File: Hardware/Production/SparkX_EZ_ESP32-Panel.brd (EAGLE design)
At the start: 187.2 x 95.5 mm, 1506 parts, among them Q1 MBT3904DW1T1, Q10 MBT3904DW1T1, Q11 MBT3904DW1T1, Q12 MBT3904DW1T1, Q13 MBT3904DW1T1, Q14 MBT3904DW1T1, Q15 MBT3904DW1T1, Q16 MBT3904DW1T1, Q17 MBT3904DW1T1, Q18 MBT3904DW1T1, Q19 MBT3904DW1T1, Q2 MBT3904DW1T1, Q20 MBT3904DW1T1, Q3 MBT3904DW1T1, Q4 MBT3904DW1T1, Q5 MBT3904DW1T1, Q6 MBT3904DW1T1, Q7 MBT3904DW1T1, Q8 MBT3904DW1T1, Q9 MBT3904DW1T1, U1 MIC5219 3.3V, U10 W25QXX128MBIT-6X5-SKINNY_CENT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, U11 CP2102N, U12 MIC5219 3.3V, U13 ESP32, U14 W25QXX128MBIT-6X5-SKINNY_CENT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, U15 CP2102N, U16 MIC5219 3.3V, U17 ESP32, U18 W25QXX128MBIT-6X5-SKINNY_CENT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, U19 CP2102N, U2 ESP32, U20 MIC5219 3.3V, U21 ESP32, U22 W25QXX128MBIT-6X5-SKINNY_CENT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, U23 CP2102N, U24 MIC5219 3.3V, U25 ESP32, U26 W25QXX128MBIT-6X5-SKINNY_CENT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, U27 CP2102N, U28 MIC5219 3.3V, U29 ESP32, U3 W25QXX128MBIT-6X5-SKINNY_CENT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, U30 W25QXX128MBIT-6X5-SKINNY_CENT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, U31 CP2102N, U32 MIC5219 3.3V, U33 ESP32, U34 W25QXX128MBIT-6X5-SKINNY_CENT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, U35 CP2102N, U36 MIC5219 3.3V, U37 ESP32, U38 W25QXX128MBIT-6X5-SKINNY_CENT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, U39 CP2102N, U4 CP2102N, U40 MIC5219 3.3V, U41 ESP32, U42 W25QXX128MBIT-6X5-SKINNY_CENT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, U43 CP2102N, U44 MIC5219 3.3V, U45 ESP32, U46 W25QXX128MBIT-6X5-SKINNY_CENT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, U47 CP2102N, U48 MIC5219 3.3V, U49 ESP32, U5 ESP32, U50 W25QXX128MBIT-6X5-SKINNY_CENT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, U51 CP2102N, U52 MIC5219 3.3V, U53 ESP32, U54 W25QXX128MBIT-6X5-SKINNY_CENT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, U55 CP2102N, U56 MIC5219 3.3V, U57 ESP32, U58 W25QXX128MBIT-6X5-SKINNY_CENT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, U59 CP2102N, U6 W25QXX128MBIT-6X5-SKINNY_CENT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, U60 MIC5219 3.3V, U61 ESP32, U62 W25QXX128MBIT-6X5-SKINNY_CENT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, U63 CP2102N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

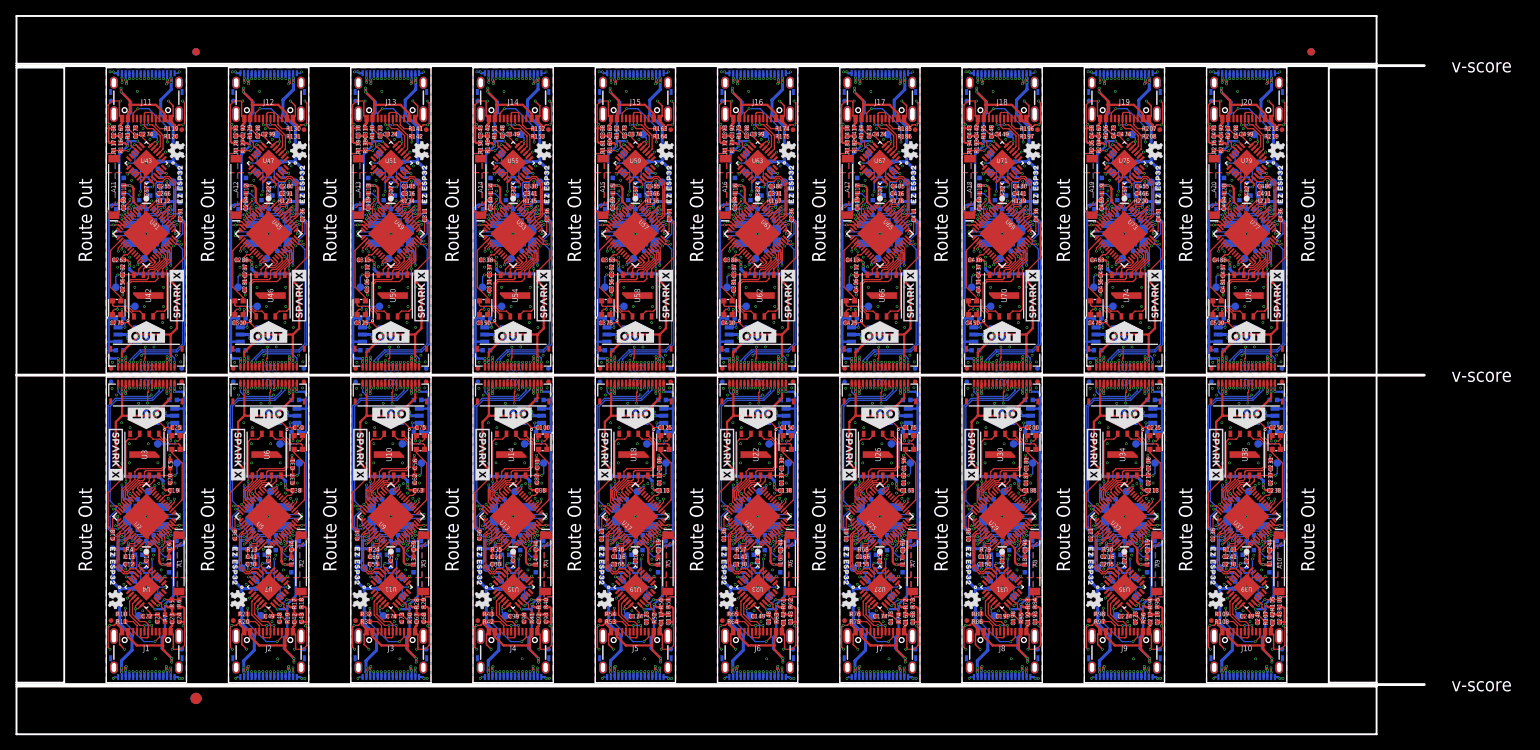
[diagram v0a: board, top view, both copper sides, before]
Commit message: Post-review updates
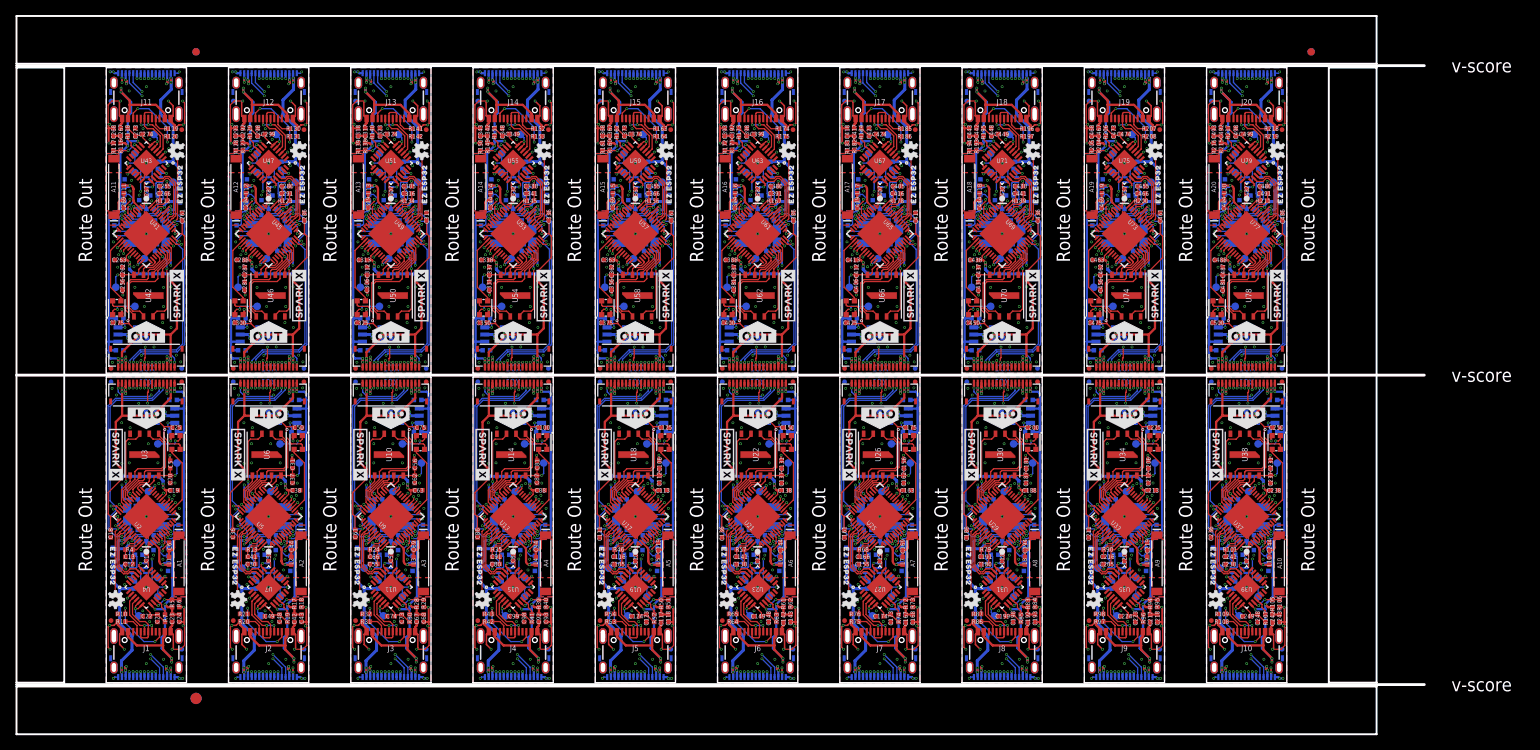
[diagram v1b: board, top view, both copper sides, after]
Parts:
- C1, C122, C147, C172, C197, C222, C247, C272, C297, C322, C347, C372, C397, C422, C447, C47, C472, C497, C72, C97: value 0.1uF -> 2.2uF
- moved C204 1.17 mm to (139.6, 20.5)
- moved C229 1.17 mm to (155.9, 20.5)
- moved C179 1.17 mm to (123.4, 20.5)
- moved C329 1.17 mm to (49.8, 61.3)
- moved C354 1.17 mm to (66.1, 61.3)
- moved C379 1.17 mm to (82.4, 61.3)
- moved C404 1.17 mm to (98.6, 61.3)
- moved C429 1.17 mm to (114.9, 61.3)
- moved C279 1.17 mm to (17.3, 61.3)
- moved C29 1.17 mm to (25.8, 20.5)
- moved C254 1.17 mm to (1.08, 61.3)
- moved C11 1.17 mm to (9.59, 20.5)
- moved C304 1.17 mm to (33.6, 61.3)
- moved C54 1.17 mm to (42.1, 20.5)
- moved C79 1.17 mm to (58.4, 20.5)
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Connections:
- net CS1: now also U2.17; no longer U2.15
- net CS10: now also U13.17; no longer U13.15
- net CS11: now also U13.20; no longer U13.16
- net CS13: now also U17.17; no longer U17.15
- net CS14: now also U17.20; no longer U17.16
- net CS16: now also U21.17; no longer U21.15
- net CS17: now also U21.20; no longer U21.16
- net CS19: now also U25.17; no longer U25.15
- net CS2: now also U2.20; no longer U2.16
- net CS20: now also U25.20; no longer U25.16
- net CS22: now also U29.17; no longer U29.15
- net CS23: now also U29.20; no longer U29.16
- net CS25: now also U33.17; no longer U33.15
- net CS26: now also U33.20; no longer U33.16
- net CS28: now also U37.17; no longer U37.15
- net CS29: now also U37.20; no longer U37.16
- net CS31: now also U41.17; no longer U41.15
- net CS32: now also U41.20; no longer U41.16
- net CS34: now also U45.17; no longer U45.15
- net CS35: now also U45.20; no longer U45.16
- net CS37: now also U49.17; no longer U49.15
- net CS38: now also U49.20; no longer U49.16
- net CS4: now also U5.17; no longer U5.15
- net CS40: now also U53.17; no longer U53.15
- net CS41: now also U53.20; no longer U53.16
- net CS43: now also U57.17; no longer U57.15
- net CS44: now also U57.20; no longer U57.16
- net CS46: now also U61.17; no longer U61.15
- net CS47: now also U61.20; no longer U61.16
- net CS49: now also U65.17; no longer U65.15
- net CS5: now also U5.20; no longer U5.16
- net CS50: now also U65.20; no longer U65.16
- net CS52: now also U69.17; no longer U69.15
- net CS53: now also U69.20; no longer U69.16
- net CS55: now also U73.17; no longer U73.15
- net CS56: now also U73.20; no longer U73.16
- net CS58: now also U77.17; no longer U77.15
- net CS59: now also U77.20; no longer U77.16
- net CS7: now also U9.17; no longer U9.15
- net CS8: now also U9.20; no longer U9.16
- net GPIO0: now also U2.16; no longer U2.10
- net GPIO1: now also U2.15; no longer U2.11
- net GPIO10: now also U21.16; no longer U21.10
- net GPIO11: now also U21.15; no longer U21.11
- net GPIO12: now also U25.16; no longer U25.10
- net GPIO13: now also U25.15; no longer U25.11
- net GPIO14: now also U29.16; no longer U29.10
- net GPIO15: now also U29.15; no longer U29.11
- net GPIO16: now also U33.16; no longer U33.10
- net GPIO17: now also U33.15; no longer U33.11
- net GPIO18: now also U37.16; no longer U37.10
- net GPIO19: now also U37.15; no longer U37.11
- net GPIO2: now also U5.16; no longer U5.10
- net GPIO20: now also U41.16; no longer U41.10
- net GPIO21: now also U41.15; no longer U41.11
- net GPIO22: now also U45.16; no longer U45.10
- net GPIO23: now also U45.15; no longer U45.11
- net GPIO24: now also U49.16; no longer U49.10
- net GPIO25: now also U49.15; no longer U49.11
- net GPIO26: now also U53.16; no longer U53.10
- net GPIO27: now also U53.15; no longer U53.11
- net GPIO28: now also U57.16; no longer U57.10
- net GPIO29: now also U57.15; no longer U57.11
- net GPIO3: now also U5.15; no longer U5.11
- net GPIO30: now also U61.16; no longer U61.10
- net GPIO31: now also U61.15; no longer U61.11
- net GPIO32: now also U65.16; no longer U65.10
- net GPIO33: now also U65.15; no longer U65.11
- net GPIO34: now also U69.16; no longer U69.10
- net GPIO35: now also U69.15; no longer U69.11
- net GPIO36: now also U73.16; no longer U73.10
- net GPIO37: now also U73.15; no longer U73.11
- net GPIO38: now also U77.16; no longer U77.10
- net GPIO39: now also U77.15; no longer U77.11
- net GPIO4: now also U9.16; no longer U9.10
- net GPIO5: now also U9.15; no longer U9.11
- net GPIO6: now also U13.16; no longer U13.10
- net GPIO7: now also U13.15; no longer U13.11
- net GPIO8: now also U17.16; no longer U17.10
- net GPIO9: now also U17.15; no longer U17.11
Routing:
- net SDA9: track 69.7 -> 50.0 mm
- net SDA8: track 69.7 -> 50.0 mm
- net SDA4: track 69.7 -> 50.0 mm
- net SDA13: track 69.7 -> 50.0 mm
- net SDA12: track 69.7 -> 50.0 mm
- net SDA1: track 69.7 -> 50.0 mm
- net SDA: track 69.7 -> 50.0 mm
- net SDA11: track 69.7 -> 50.0 mm
- net SDA10: track 69.7 -> 50.0 mm
- net SDA3: track 69.7 -> 50.0 mm
- net SDA2: track 69.7 -> 50.0 mm
- net SDA17: track 69.7 -> 50.0 mm
- net SDA16: track 69.7 -> 50.0 mm
- net SDA15: track 69.7 -> 50.0 mm
- net SDA14: track 69.7 -> 50.0 mm
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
